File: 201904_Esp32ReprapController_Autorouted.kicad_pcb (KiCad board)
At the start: 2 copper layers, 157.5 x 97.8 mm, 62 parts, among them J1 - 24V_IN +, J10 + NOZZLE -, J11 + BED -, J110 MOTOR_X, J12 + FAN1 -, J120 MOTOR_Y, J13 + FAN2 -, J130 MOTOR_Z, J14 + FAN3 -, J140 MOTOR_E, J20 + BED_T -, J21 + NOZ_T -, J30 + X_Min -, J31 + Y_Min -, J32 + Z_Min -, J40 LCD, J50 SD_Card GND, J60 BLTouch, Q1 IRLZ44N, Q2 IRLB8743, U1 ESP32-DEVKITC-32D, U2 DcStepDown_LM2596, U3 74HC595, U4 74HC595, U5 ULN2803A

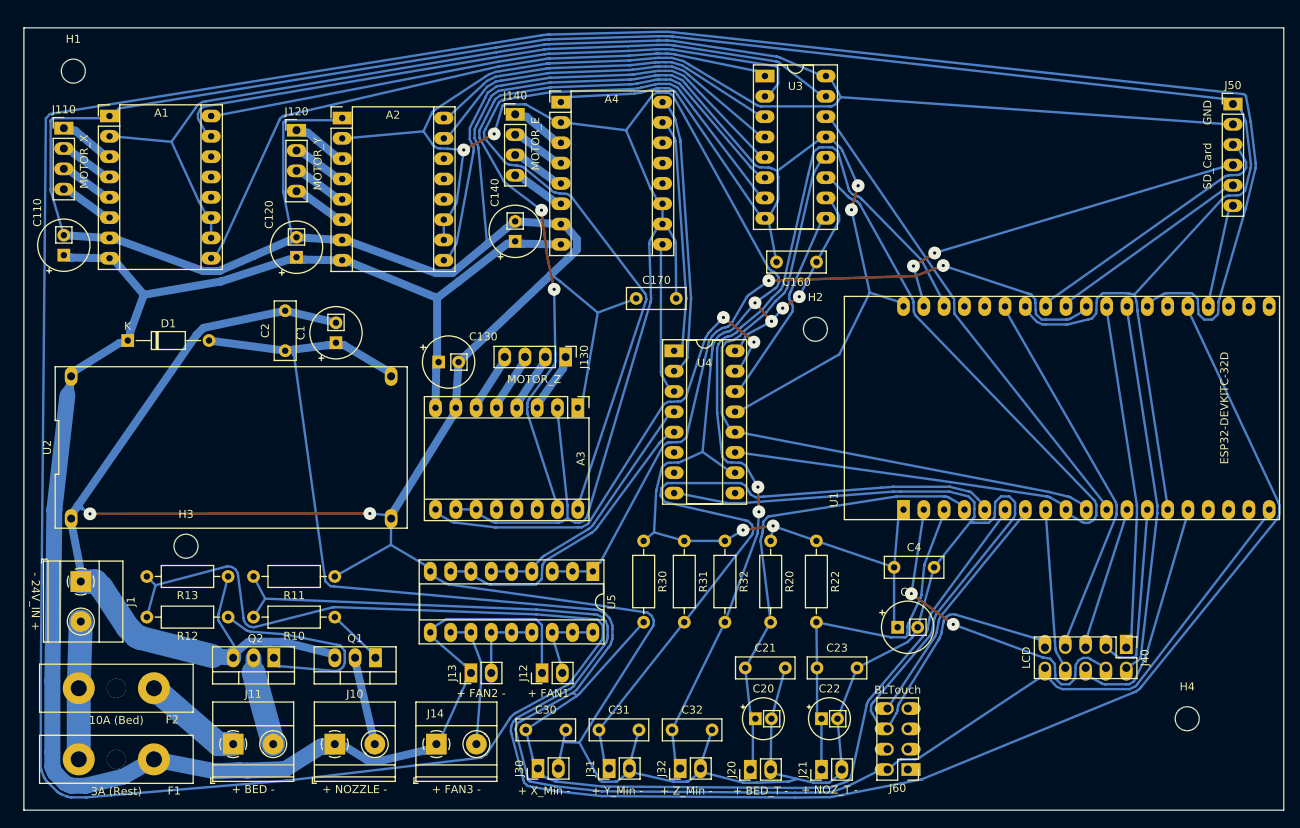
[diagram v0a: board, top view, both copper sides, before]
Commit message: board r3 (milled and built 2019-06)
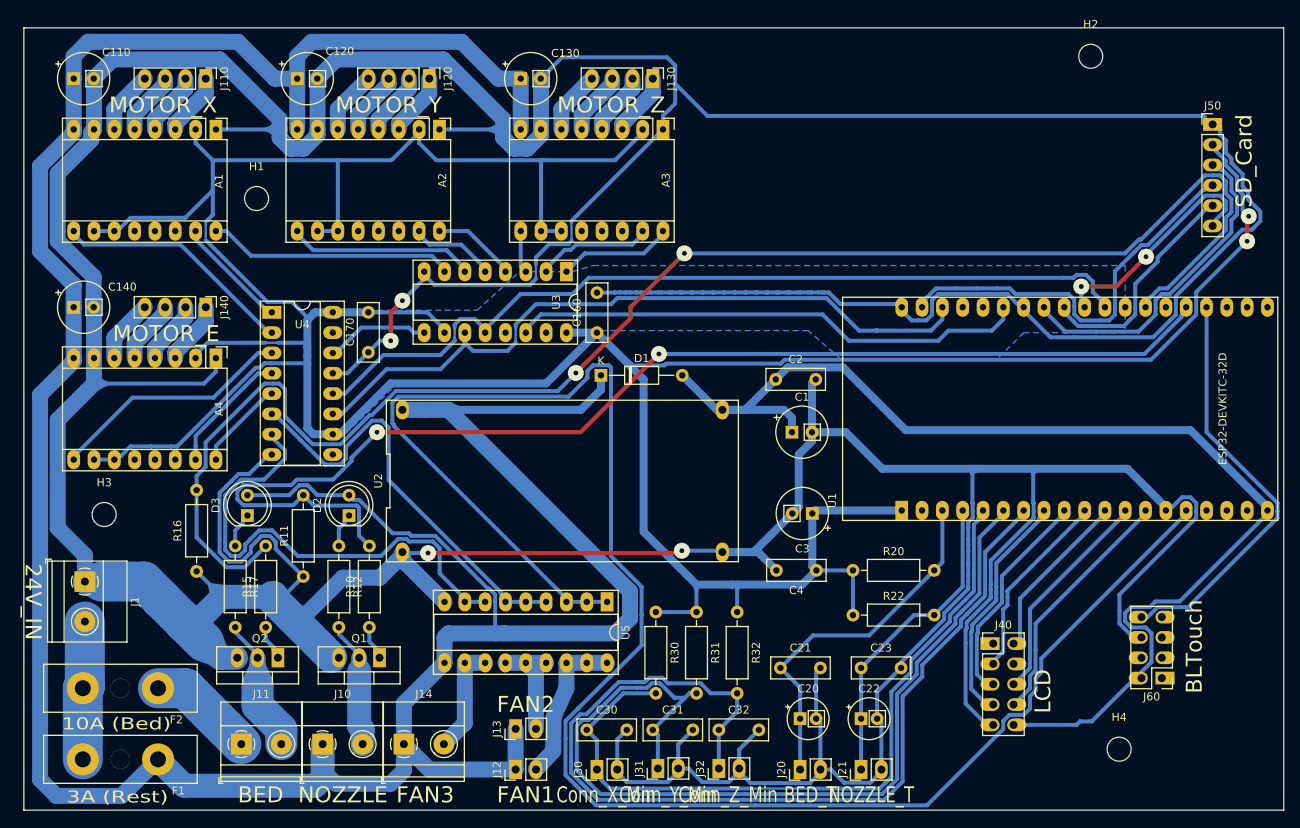
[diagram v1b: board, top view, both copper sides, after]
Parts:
- removed R13: 100k, Felix_Common:R_Axial_DIN0207_L6.3mm_D2.5mm_P10.16mm_Horizontal
- added D2: LED_NOZ, Felix_Common:LED_D5.0mm, F.Cu at (66.0, 90.2)
- added D3: LED_BED, Felix_Common:LED_D5.0mm, F.Cu at (53.3, 90.2)
- added R15: 10, Felix_Common:R_Axial_DIN0207_L6.3mm_D2.5mm_P10.16mm_Horizontal, F.Cu at (55.6, 104.1)
- added R16: 100k, Felix_Common:R_Axial_DIN0207_L6.3mm_D2.5mm_P10.16mm_Horizontal, F.Cu at (47.0, 97.2)
- added R17: 2.2k, Felix_Common:R_Axial_DIN0207_L6.3mm_D2.5mm_P10.16mm_Horizontal, F.Cu at (51.8, 94.0)
- J1: value - 24V_IN + -> 24V_IN
- J10: value + NOZZLE - -> NOZZLE
- J11: value + BED - -> BED
- J12: value + FAN1 - -> FAN1
- J13: value + FAN2 - -> FAN2
- J14: value + FAN3 - -> FAN3
- J20: value + BED_T - -> BED_T
- J21: value + NOZ_T - -> NOZZLE_T
- J30: value + X_Min - -> Conn_X_Min
- J31: value + Y_Min - -> Conn_Y_Min
- J32: value + Z_Min - -> Conn_Z_Min
- J50: value SD_Card GND -> SD_Card
- R12: value 10 -> 2.2k
- moved C2 61.4 mm to (119.4, 73.2), turned to 0 degrees
- moved D1 59.3 mm to (97.5, 72.6)
- moved C1 58.1 mm to (121.4, 79.8), turned to 0 degrees
- moved C140 55.8 mm to (31.6, 64.1), turned to 0 degrees
- moved A4 53.7 mm to (49.4, 70.5), turned to 270 degrees
- moved U4 50.5 mm to (56.4, 64.8)
- moved H2 48.5 mm to (158.8, 32.8)
- moved J140 45.6 mm to (48.1, 64.1), turned to 270 degrees
- moved U2 41.6 mm to (92.7, 85.9)
- moved C170 38.5 mm to (68.5, 64.8), turned to 270 degrees
- moved C130 36.9 mm to (87.5, 35.6)
- moved J130 36.5 mm to (104.0, 35.6)
- moved A3 36.4 mm to (105.3, 41.9)
- moved U3 34.8 mm to (93.2, 59.7), turned to 270 degrees
- moved J60 33.7 mm to (167.6, 110.5)
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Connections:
- net /FAN1 renamed /IO13_FAN1
- net /NOZZLE renamed /IO2_NOZZLE
- net /Q132 renamed /Q132_Y_DIR
- net /Q139 renamed /Q139_E_EN
- net /X_MIN renamed /IO34_X_MIN
- net /Y_MIN renamed /IO35_Y_MIN
- A1 pad 15: /Q128 -> /Q137_X_STEP
- A1 pad 16: /Q129 -> /Q135_X_DIR
- A1 pad 9: /Q130 -> /Q138_X_EN
- A2 pad 15: /Q131 -> /Q133_Y_STEP
- A2 pad 9: /Q133 -> /Q134_Y_EN
- A3 pad 15: /Q134 -> /Q130_Z_STEP
- A3 pad 16: /Q135 -> /Q129_Z_DIR
- A3 pad 9: /Q136 -> /Q131_Z_EN
- A4 pad 15: /Q137 -> /Q140_E_STEP
- A4 pad 16: /Q138 -> /Q141_E_DIR
- C20 pad 1: /BED_T -> /I36_T_BED
- C21 pad 1: /BED_T -> /I36_T_BED
- C22 pad 1: /NOZZLE_T -> /I39_T_NOZ
- C23 pad 1: /NOZZLE_T -> /I39_T_NOZ
- C32 pad 1: /Z_MIN -> /IO32_Z_MIN
- J20 pad 1: /BED_T -> /I36_T_BED
- J21 pad 1: /NOZZLE_T -> /I39_T_NOZ
- J32 pad 1: /Z_MIN -> /IO32_Z_MIN
- J40 pad 2: /BTN_ENC -> /IO27_BTN_ENC
- J40 pad 3: /BTN_EN1 -> /IO26_BTN_EN1
- J40 pad 5: /BTN_EN2 -> /IO25_BTN_EN2
- J40 pad 6: /LCD_D4 -> /IO14_LCD_D4
- J40 pad 7: /LCD_RS -> /IO33_LCD_RS
- J40 pad 8: /LCD_EN -> /IO12_LCD_EN
- J60 pad 8: /SERVO -> /IO15_SERVO
- R12 pad 1: Net-(Q2-Pad1) -> Net-(D2-Pad1)
- R12 pad 2: /BED -> Net-(J10-Pad2)
- R20 pad 2: /BED_T -> /I36_T_BED
- R22 pad 2: /NOZZLE_T -> /I39_T_NOZ
- R32 pad 2: /Z_MIN -> /IO32_Z_MIN
- U1 pad 10: /I2S_WS -> /IO26_BTN_EN1
- U1 pad 11: /I2S_DATA -> /IO27_BTN_ENC
- U1 pad 12: /BTN_EN2 -> /IO14_LCD_D4
- U1 pad 13: /BTN_EN1 -> /IO12_LCD_EN
- U1 pad 2: /~RESET -> /~ESP32_EN
- U1 pad 22: /LCD_D4 -> /IO22_I2S_BCK
- U1 pad 25: /LCD_EN -> /IO21_I2S_DATA
- U1 pad 3: /NOZZLE_T -> /I36_T_BED
- U1 pad 30: /LCD_RS -> /IO17_I2S_WS
- U1 pad 31: /BEEPER -> Net-(U1-Pad31)
- U1 pad 32: /BED -> /IO4_BED
- U1 pad 35: /Z_MIN -> /IO15_SERVO
- U1 pad 4: /BED_T -> /I39_T_NOZ
- U1 pad 7: /SERVO -> /IO32_Z_MIN
- U1 pad 8: /BTN_ENC -> /IO33_LCD_RS
- U1 pad 9: /I2S_BCK -> /IO25_BTN_EN2
- U3 pad 1: /Q129 -> /Q129_Z_DIR
- U3 pad 11: /I2S_BCK -> /IO22_I2S_BCK
- U3 pad 12: /I2S_WS -> /IO17_I2S_WS
- U3 pad 14: /I2S_DATA -> /IO21_I2S_DATA
- U3 pad 2: /Q130 -> /Q130_Z_STEP
- U3 pad 3: /Q131 -> /Q131_Z_EN
- U3 pad 5: /Q133 -> /Q133_Y_STEP
- U3 pad 6: /Q134 -> /Q134_Y_EN
- U3 pad 7: /Q135 -> /Q135_X_DIR
- U4 pad 1: /Q137 -> /Q137_X_STEP
- U4 pad 11: /I2S_BCK -> /IO22_I2S_BCK
- U4 pad 12: /I2S_WS -> /IO17_I2S_WS
- U4 pad 2: /Q138 -> /Q138_X_EN
- U4 pad 4: /Q140 -> /Q140_E_STEP
- U4 pad 5: /Q141 -> /Q141_E_DIR
- U4 pad 6: /Q142 -> /Q142_FAN2
- U4 pad 7: /Q143 -> /Q143_FAN3
- U5 pad 4: /Q140 -> /Q142_FAN2
- U5 pad 5: /Q140 -> /Q142_FAN2
- U5 pad 6: /Q140 -> /Q142_FAN2
- U5 pad 7: /Q141 -> /Q143_FAN3
- U5 pad 8: /Q141 -> /Q143_FAN3
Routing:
- net /BED: track 422.0 -> 0.00 mm
- net /IO4_BED: track 0.00 -> 195.4 mm, vias 0 -> 2
- net +24V: track 238.9 -> 401.7 mm
- net /IO13_FAN1: track 93.3 -> 223.5 mm, vias 2 -> 0
- net /IO32_Z_MIN: track 0.00 -> 124.4 mm
- net /Z_MIN: track 114.0 -> 0.00 mm, vias 2 -> 0
- net /IO17_I2S_WS: track 0.00 -> 108.9 mm
- net /I2S_BCK: track 102.7 -> 0.00 mm
- net /Q135: track 102.6 -> 0.00 mm
- net /Q134: track 96.2 -> 0.00 mm, vias 2 -> 0
- net GND: track 997.5 -> 904.1 mm
- net /IO22_I2S_BCK: track 0.00 -> 92.0 mm
- net /I2S_WS: track 85.4 -> 0.00 mm
- net /Q128: track 84.7 -> 0.00 mm
- net /Q130: track 81.6 -> 0.00 mm
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- added copper zone on B.Cu, net GND
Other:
- net class Default: clearance 0.2 -> 0.18; trace_width 0.3 -> 0.5; via_dia 0.8 -> 2; via_drill 0.4 -> 0.6
- rule trace_clearance: 0.2 -> 0.18
- rule trace_min: 0.18 -> 0.3
